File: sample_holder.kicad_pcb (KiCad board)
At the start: 4 copper layers, 50 x 50 mm, 14 parts, among them J1 Conn_Coaxial, J10 RF_Shield_One_Piece, J2 Conn_Coaxial, J3 Conn_Coaxial, J4 Conn_Coaxial, J5 Conn_Coaxial, J6 Conn_Coaxial, J7 Conn_Coaxial, J8 Conn_Coaxial, U1 sample

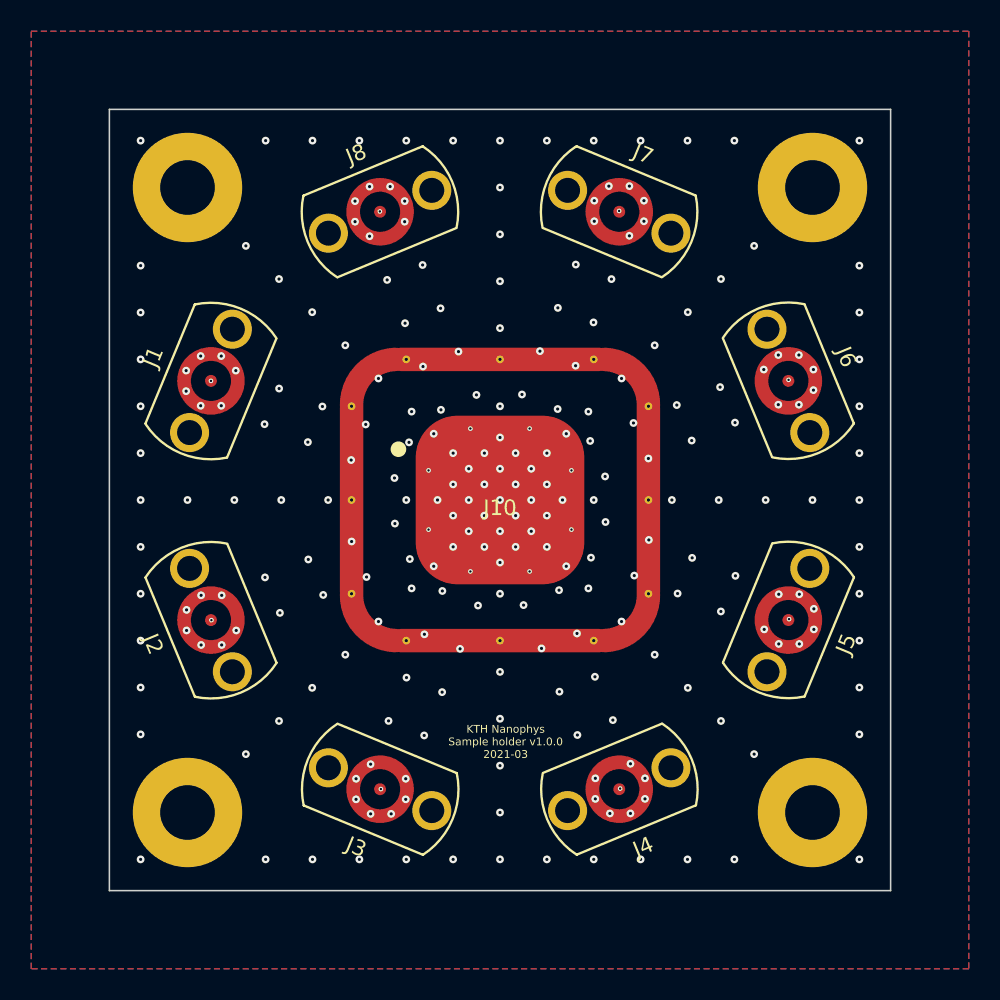
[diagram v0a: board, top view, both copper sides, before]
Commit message: Update sample_holder.kicad_pcb, sample_holder.pro, and stackup.txt
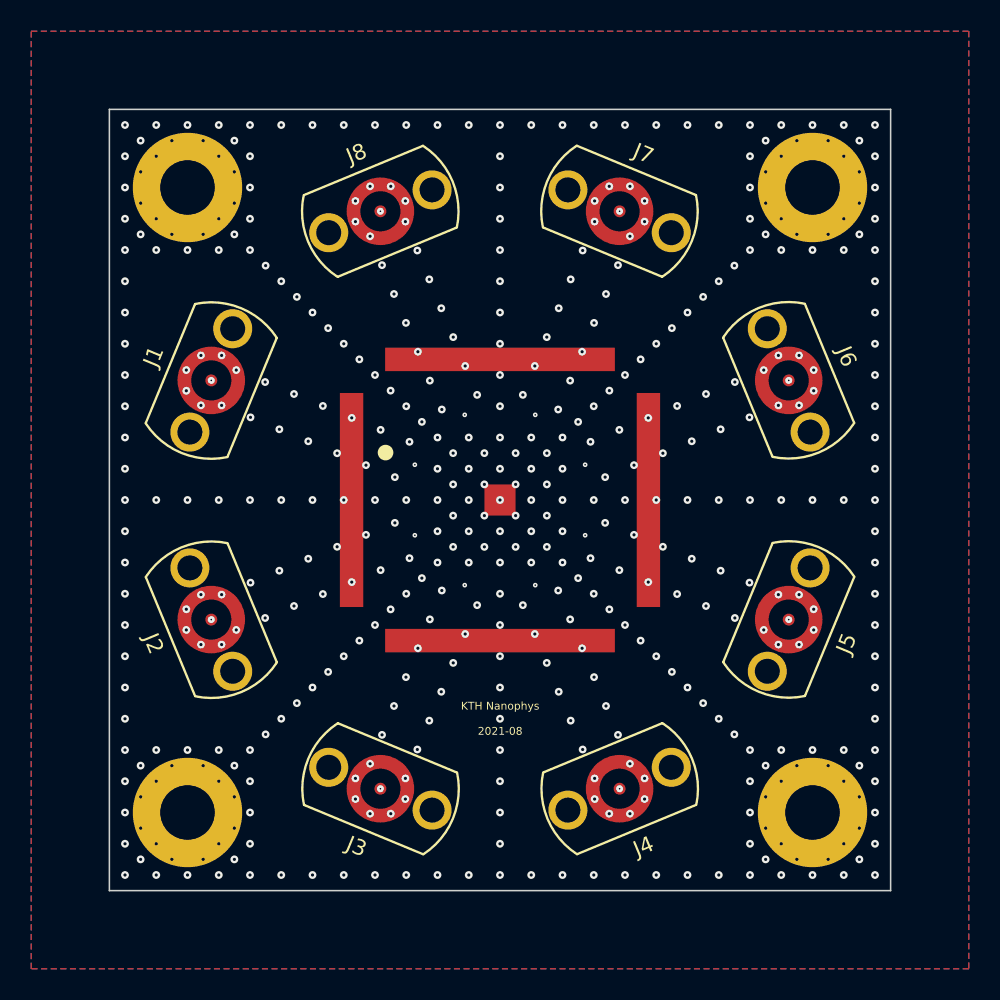
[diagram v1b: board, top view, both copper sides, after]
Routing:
- net Net-(J8-Pad1): track 15.1 -> 14.1 mm
- net Net-(J6-Pad1): track 15.1 -> 14.1 mm
- net Net-(J4-Pad1): track 15.1 -> 14.1 mm
- net Net-(J2-Pad1): track 15.1 -> 14.1 mm
- net Net-(J7-Pad1): track 15.1 -> 14.1 mm
- net Net-(J5-Pad1): track 15.1 -> 14.1 mm
- net Net-(J3-Pad1): track 15.1 -> 14.1 mm
- net Net-(J1-Pad1): track 15.1 -> 14.1 mm
- net GND: vias 245 -> 461
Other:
- net class Traces: clearance 0.54 -> 0.3; trace_width 0.31642 -> 0.281959
- rule via_min_drill: 0.15 -> 0.1
- board text added: "KTH Nanophys 2021-08"
- board text removed: "KTH Nanophys Sample holder v1.0.0 2021-03"

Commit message: fix up libraries
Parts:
- J1, J2, J3, J4, J5, J6, J7, J8: footprint imp:0732513481 -> sample_holder:0732513481
